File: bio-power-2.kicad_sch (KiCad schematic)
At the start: 45 parts, among them J1 USB_C_Receptacle, J2 6vdc, J3 6.5V, U1 STUSB4500QTR, U2 TPS5430DDA, U3 LT3041ADE-PBF

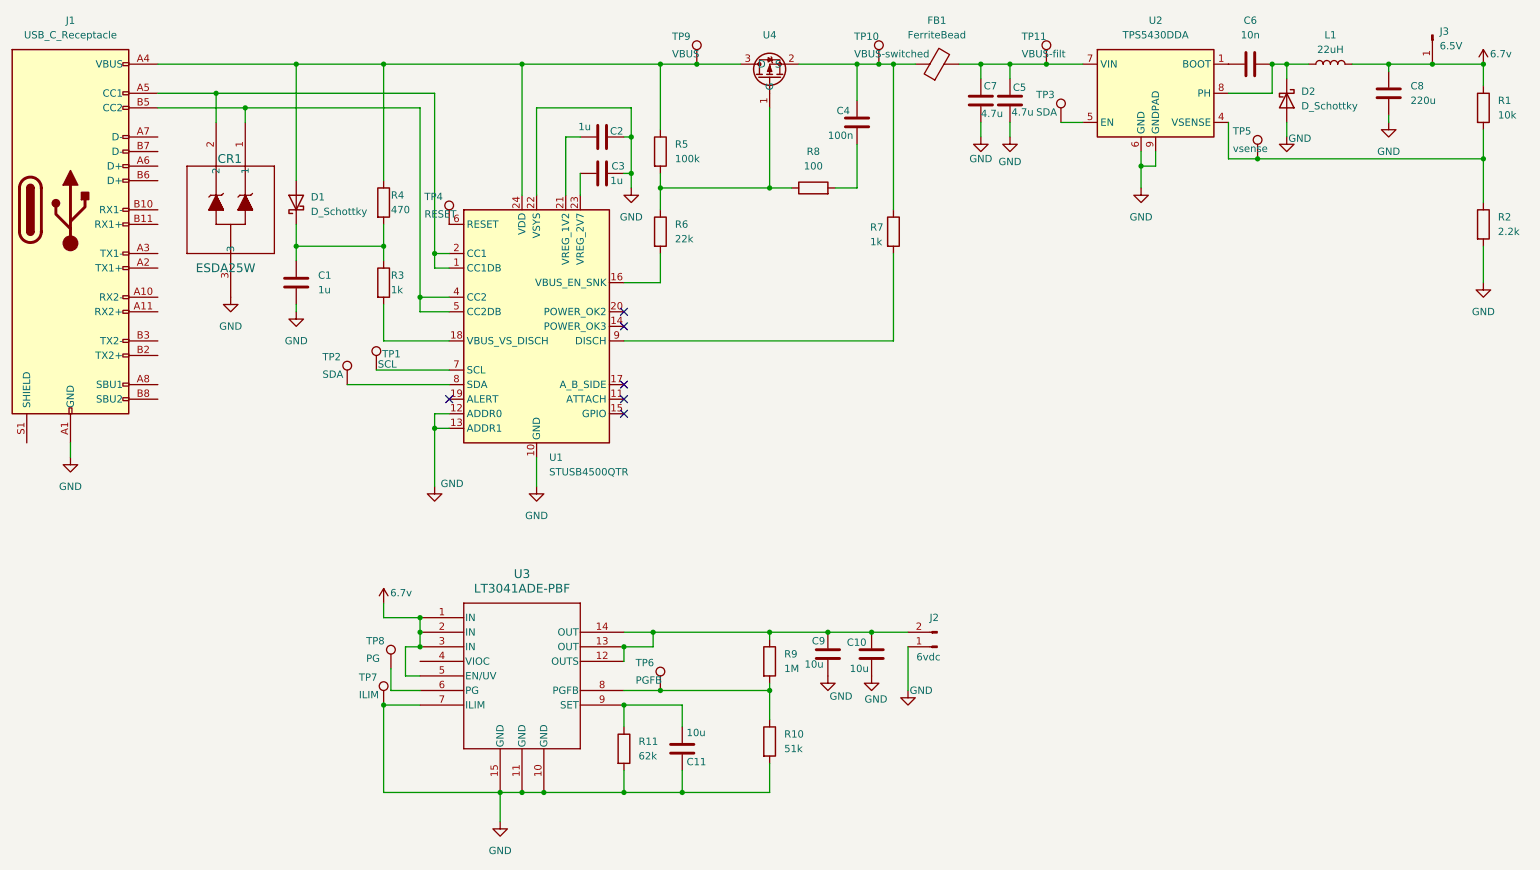
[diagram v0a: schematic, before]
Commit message: new symbols
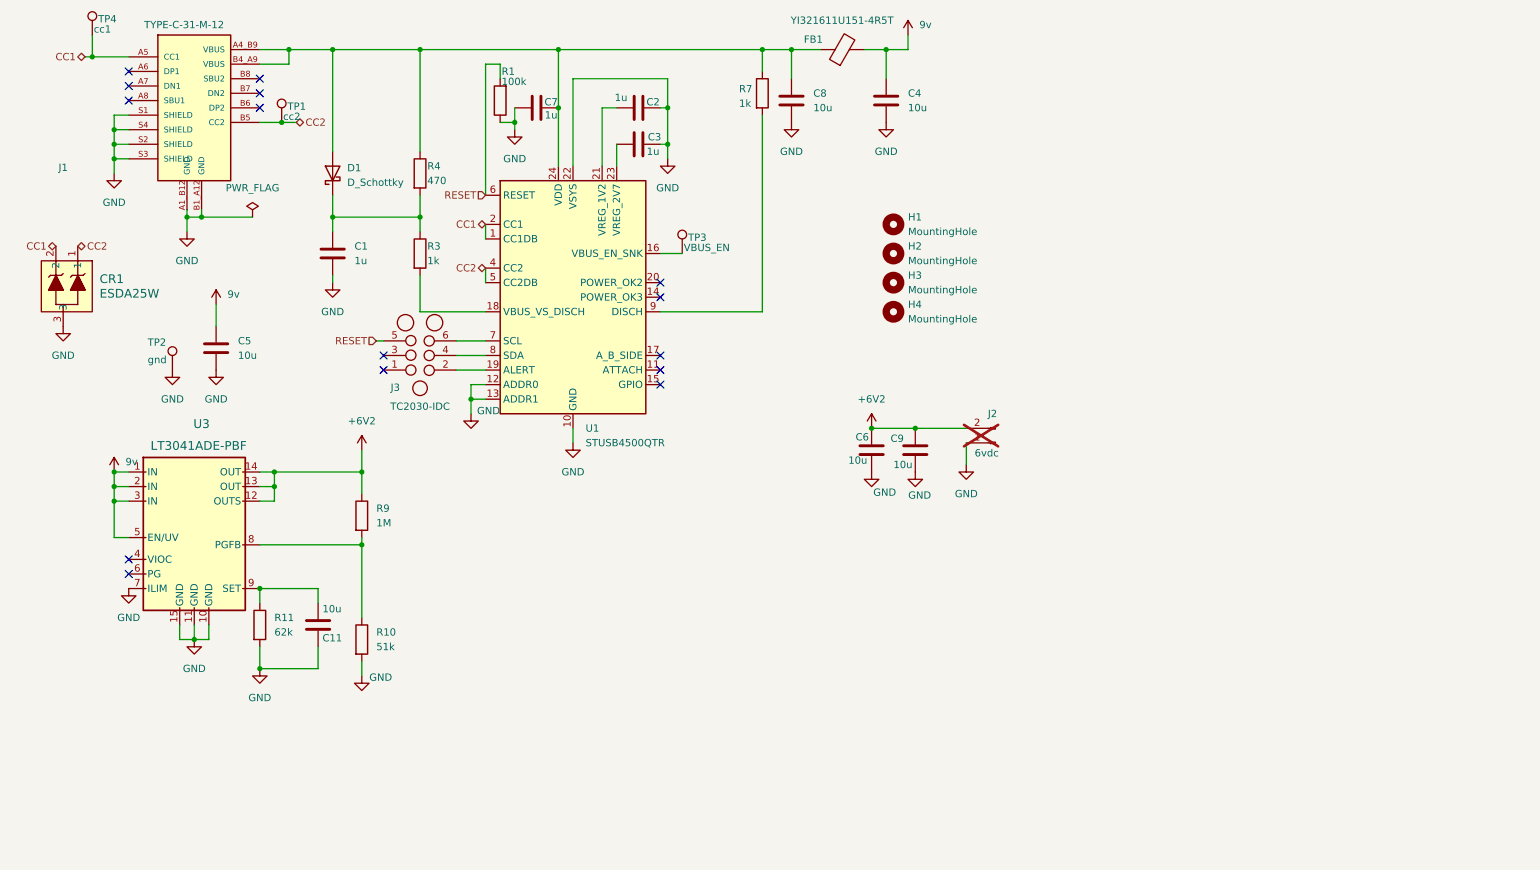
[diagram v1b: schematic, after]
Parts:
- removed C10: 10u, symbol Device:C
- removed CR1: ESDA25W, SOT323-3L_STM, symbol 2024-06-03_16-24-40:ESDA25W
- removed D2: D_Schottky, symbol Device:D_Schottky
- removed J1: USB_C_Receptacle, Connector_USB:USB_C_Plug_Molex_105444, symbol Connector:USB_C_Receptacle
- removed J3: 6.5V, symbol Connector:Conn_01x01_Pin
- removed L1: 22uH, symbol Device:L
- removed R2: 2.2k, symbol Device:R
- removed R5: 100k, Resistor_SMD:R_0805_2012Metric, symbol Device:R
- removed R6: 22k, Resistor_SMD:R_0805_2012Metric, symbol Device:R
- removed R8: 100, Resistor_SMD:R_0805_2012Metric, symbol Device:R
- removed TP10: VBUS-switched, TestPoint:TestPoint_Pad_D3.0mm, symbol Connector:TestPoint
- removed TP11: VBUS-filt, TestPoint:TestPoint_Pad_D3.0mm, symbol Connector:TestPoint
- removed TP5: vsense, TestPoint:TestPoint_Pad_D3.0mm, symbol Connector:TestPoint
- removed TP6: PGFB, TestPoint:TestPoint_Pad_D3.0mm, symbol Connector:TestPoint
- removed TP7: ILIM, TestPoint:TestPoint_Pad_D3.0mm, symbol Connector:TestPoint
- removed TP8: PG, TestPoint:TestPoint_Pad_D3.0mm, symbol Connector:TestPoint
- removed TP9: VBUS, TestPoint:TestPoint_Pad_D3.0mm, symbol Connector:TestPoint
- removed U2: TPS5430DDA, Package_SO:TI_SO-PowerPAD-8_ThermalVias, symbol Regulator_Switching:TPS5430DDA
- removed U4: ~, Package_TO_SOT_SMD:SOT-23, symbol mosfet:hl2301a
- added CR1: ESDA25W, footprints:SOT323-3L_STM, symbol tvs_esda:ESDA25W
- added H1, H2, H3, H4: MountingHole, MountingHole:MountingHole_2.5mm, symbol Mechanical:MountingHole
- added J1: TYPE-C-31-M-12, typec:HRO_TYPE-C-31-M-12, symbol TYPE-C-31-M-12:TYPE-C-31-M-12
- added J3: TC2030-IDC, Tag-Connect:Tag-Connect_TC2030-IDC-NL_2x03_P1.27mm_Vertical, symbol Tag-Connect:TC2030-IDC
- C1, C2, C3: footprint (none) -> Capacitor_SMD:C_0402_1005Metric; jlcpcb (none) -> C52923
- C11, C9: footprint (none) -> Capacitor_SMD:C_0603_1608Metric; jlcpcb (none) -> C96446
- C4: value 100n -> 10u; footprint (none) -> Capacitor_SMD:C_0603_1608Metric; jlcpcb (none) -> C96446
- C5: value 4.7u -> 10u; footprint (none) -> Capacitor_SMD:C_0603_1608Metric; jlcpcb (none) -> C96446
- C6: value 10n -> 10u; footprint (none) -> Capacitor_SMD:C_0603_1608Metric; jlcpcb (none) -> C96446
- C7: value 4.7u -> 1u; footprint (none) -> Capacitor_SMD:C_0402_1005Metric; jlcpcb (none) -> C52923
- C8: value 220u -> 10u; footprint (none) -> Capacitor_SMD:C_0603_1608Metric; jlcpcb (none) -> C96446
- D1: footprint (none) -> Diode_SMD:D_SOD-323; jlcpcb (none) -> C7420331
- FB1: value FerriteBead -> YI321611U151-4R5T; footprint (none) -> Inductor_SMD:L_1206_3216Metric; jlcpcb (none) -> C3033918
- J2: now not fitted
- R1: value 10k -> 100k; footprint (none) -> Resistor_SMD:R_0805_2012Metric; jlcpcb (none) -> C149504
- R10: footprint (none) -> Resistor_SMD:R_0805_2012Metric; jlcpcb (none) -> C17737
- R11: footprint (none) -> Resistor_SMD:R_0805_2012Metric; jlcpcb (none) -> C17783
- R3: footprint (none) -> Resistor_SMD:R_0805_2012Metric; jlcpcb (none) -> C17513
- R4: footprint (none) -> Resistor_SMD:R_0805_2012Metric; jlcpcb (none) -> C2974575
- R7: jlcpcb (none) -> C17513
- R9: footprint (none) -> Resistor_SMD:R_0805_2012Metric; jlcpcb (none) -> C17514
- TP1: value SCL -> cc2; footprint TestPoint:TestPoint_Pad_D3.0mm -> TestPoint:TestPoint_Pad_1.0x1.0mm
- TP2: value SDA -> gnd; footprint TestPoint:TestPoint_Pad_D3.0mm -> TestPoint:TestPoint_Pad_1.0x1.0mm
- TP3: value SDA -> VBUS_EN; footprint TestPoint:TestPoint_Pad_D3.0mm -> TestPoint:TestPoint_Pad_1.0x1.0mm
- TP4: value RESET -> cc1; footprint TestPoint:TestPoint_Pad_D3.0mm -> TestPoint:TestPoint_Pad_1.0x1.0mm
- U1: footprint Package_DFN_QFN:QFN-24-1EP_4x4mm_P0.5mm_EP2.7x2.7mm -> Package_DFN_QFN:QFN-24-1EP_4x4mm_P0.5mm_EP2.15x2.15mm_ThermalVias
- U3: jlcpcb (none) -> C7452881
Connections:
- net GND: now also C4.2, C6.2, C7.1, R1.1, TP2.1, CR1.3, J1.A1_B12 (GND), J1.B1_A12 (GND), J1.S1 (SHIELD), J1.S2 (SHIELD), J1.S3 (SHIELD), J1.S4 (SHIELD); no longer C7.2
- net at D1.2 (A), R4.1, U1.24 (VDD): now also C7.2, C8.1, FB1.1, R7.1, J1.A4_B9 (VBUS), J1.B4_A9 (VBUS)
- net +6V2: now reaches C9.1, J2.2 (Pin_2), R9.1, U3.12 (OUTS), U3.13 (OUT), U3.14 (OUT)
- net +6V2: now also C6.1
- net RESET: now reaches R1.2
- net RESET: now also U1.6 (RESET), J3.5 (Pin_5)
- net 9v: now reaches C5.1, FB1.2
- net 9v: now also C4.1, U3.1 (IN), U3.2 (IN), U3.3 (IN), U3.5 (EN/UV); no longer C7.1
- net at TP3.1: now also U1.16 (VBUS_EN_SNK)
- net CC2: now reaches U1.4 (CC2), U1.5 (CC2DB)
- net CC2: now also TP1.1, CR1.1, J1.B5 (CC2)
- net CC1: now reaches U1.1 (CC1DB), U1.2 (CC1)
- net CC1: now also TP4.1, CR1.2, J1.A5 (CC1)
- net at U1.8 (SDA): now also J3.4 (Pin_4); no longer TP2.1
- net at U1.19 (ALERT): now also J3.2 (Pin_2)
- net at U1.7 (SCL): now also J3.6 (Pin_6); no longer TP1.1
- removed net 6.7v: C8.1, R1.1, U3.1 (IN), U3.2 (IN), U3.3 (IN), U3.5 (EN/UV)
- no-connect marks 6 -> 15
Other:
- company: (none) -> Utrecht University
- title: (none) -> Biosemi USBC adapter
- moved on the sheet: C1, C11, C2, C3, D1, FB1, R10, R11, R3, R4, R7, R9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
